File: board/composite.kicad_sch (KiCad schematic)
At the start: 18 parts, among them J6 COMPOSITE, U17 CPST, U18 74HC373, U19 74HC373, U20 74HC165, U21 74HC165, Y1 14.318MHz

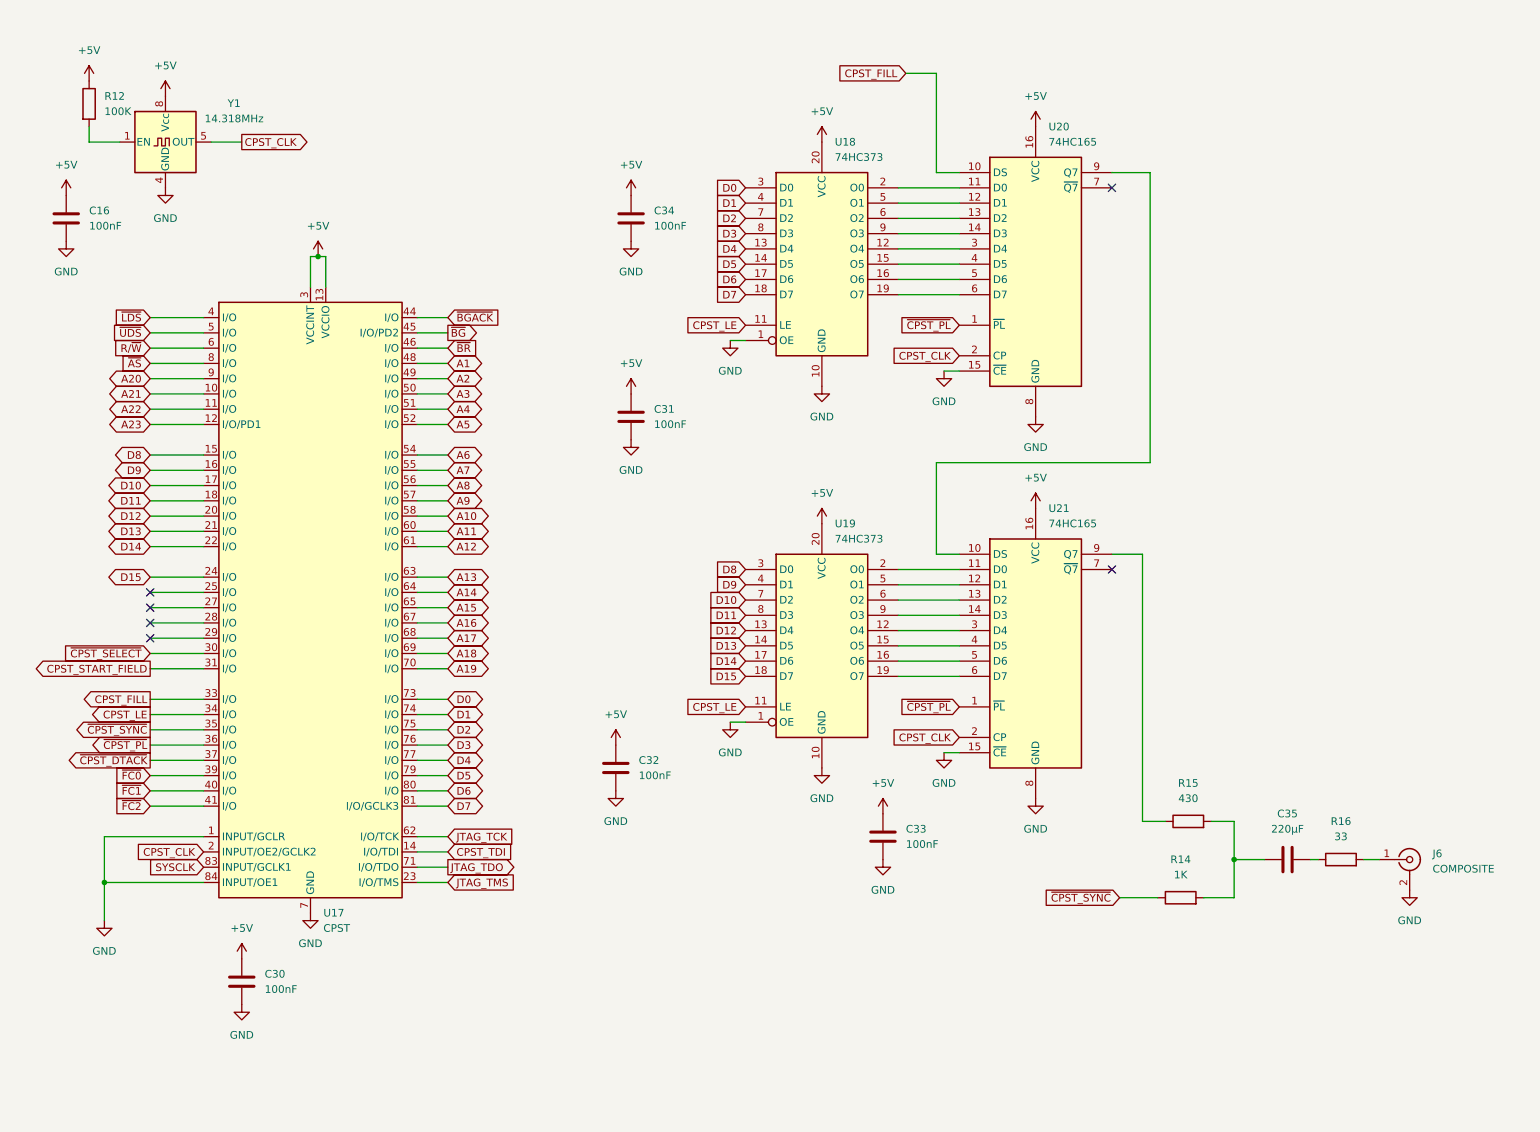
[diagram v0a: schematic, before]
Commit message: checkpoint
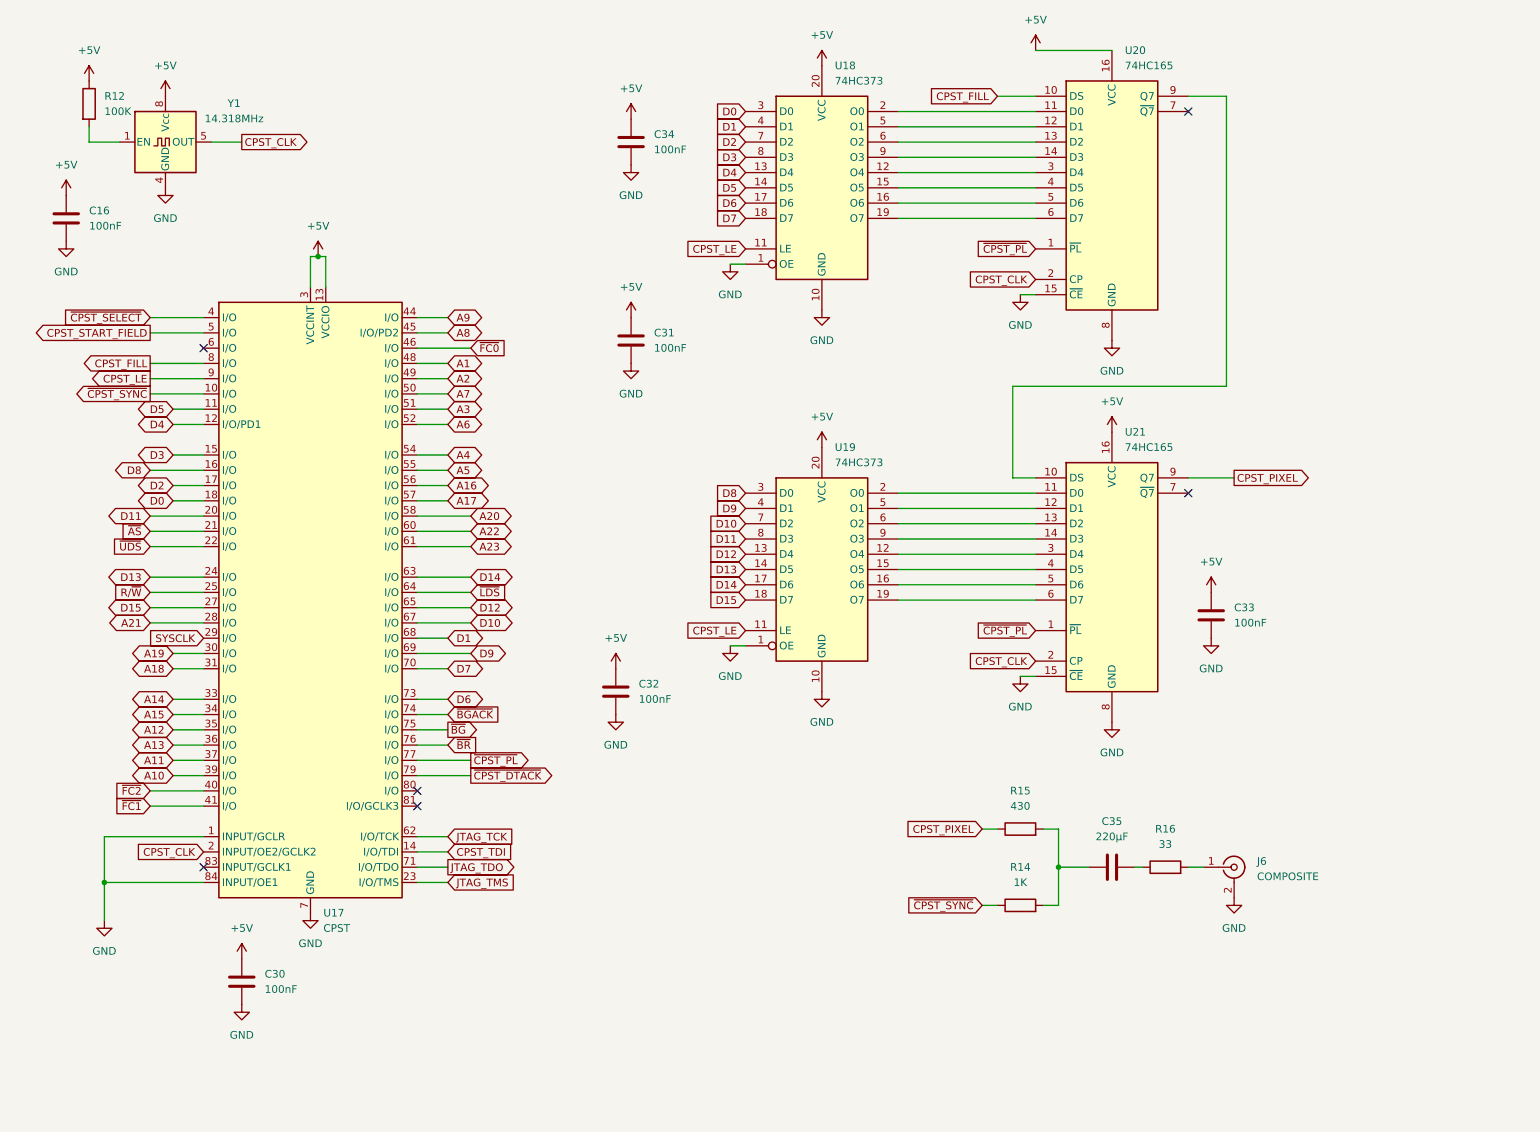
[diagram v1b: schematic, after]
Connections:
- net A10: now also U17.39 (I/O); no longer U17.58 (I/O)
- net A11: now also U17.37 (I/O); no longer U17.60 (I/O)
- net A12: now also U17.35 (I/O); no longer U17.61 (I/O)
- net A13: now also U17.36 (I/O); no longer U17.63 (I/O)
- net A14: now also U17.33 (I/O); no longer U17.64 (I/O)
- net A15: now also U17.34 (I/O); no longer U17.65 (I/O)
- net A16: now also U17.56 (I/O); no longer U17.67 (I/O)
- net A17: now also U17.57 (I/O); no longer U17.68 (I/O)
- net A18: now also U17.31 (I/O); no longer U17.69 (I/O)
- net A19: now also U17.30 (I/O); no longer U17.70 (I/O)
- net A20: now also U17.58 (I/O); no longer U17.9 (I/O)
- net A21: now also U17.28 (I/O); no longer U17.10 (I/O)
- net A22: now also U17.60 (I/O); no longer U17.11 (I/O)
- net A23: now also U17.61 (I/O); no longer U17.12 (I/O/PD1)
- net A3: now also U17.51 (I/O); no longer U17.50 (I/O)
- net A4: now also U17.54 (I/O); no longer U17.51 (I/O)
- net A5: now also U17.55 (I/O); no longer U17.52 (I/O)
- net A6: now also U17.52 (I/O); no longer U17.54 (I/O)
- net A7: now also U17.50 (I/O); no longer U17.55 (I/O)
- net A8: now also U17.45 (I/O/PD2); no longer U17.56 (I/O)
- net A9: now also U17.44 (I/O); no longer U17.57 (I/O)
- net CPST_FILL: now also U17.8 (I/O); no longer U17.33 (I/O)
- net CPST_LE: now also U17.9 (I/O); no longer U17.34 (I/O)
- net CPST_START_FIELD: now also U17.5 (I/O); no longer U17.31 (I/O)
- net D0: now also U17.18 (I/O); no longer U17.73 (I/O)
- net D1: now also U17.68 (I/O); no longer U17.74 (I/O)
- net D10: now also U17.67 (I/O); no longer U17.17 (I/O)
- net D11: now also U17.20 (I/O); no longer U17.18 (I/O)
- net D12: now also U17.65 (I/O); no longer U17.20 (I/O)
- net D13: now also U17.24 (I/O); no longer U17.21 (I/O)
- net D14: now also U17.63 (I/O); no longer U17.22 (I/O)
- net D15: now also U17.27 (I/O); no longer U17.24 (I/O)
- net D2: now also U17.17 (I/O); no longer U17.75 (I/O)
- net D3: now also U17.15 (I/O); no longer U17.76 (I/O)
- net D4: now also U17.12 (I/O/PD1); no longer U17.77 (I/O)
- net D5: now also U17.11 (I/O); no longer U17.79 (I/O)
- net D6: now also U17.73 (I/O); no longer U17.80 (I/O)
- net D7: now also U17.70 (I/O); no longer U17.81 (I/O/GCLK3)
- net D8: now also U17.16 (I/O); no longer U17.15 (I/O)
- net D9: now also U17.69 (I/O); no longer U17.16 (I/O)
- net R/~{W}: now also U17.25 (I/O); no longer U17.6 (I/O)
- net SYSCLK: now also U17.29 (I/O); no longer U17.83 (INPUT/GCLK1)
- net ~{AS}: now also U17.21 (I/O); no longer U17.8 (I/O)
- net ~{BGACK}: now also U17.74 (I/O); no longer U17.44 (I/O)
- net ~{BG}: now also U17.75 (I/O); no longer U17.45 (I/O/PD2)
- net ~{BR}: now also U17.76 (I/O); no longer U17.46 (I/O)
- net ~{CPST_DTACK}: now also U17.79 (I/O); no longer U17.37 (I/O)
- net ~{CPST_PL}: now also U17.77 (I/O); no longer U17.36 (I/O)
- net ~{CPST_SELECT}: now also U17.4 (I/O); no longer U17.30 (I/O)
- net ~{CPST_SYNC}: now also U17.10 (I/O); no longer U17.35 (I/O)
- net ~{FC0}: now also U17.46 (I/O); no longer U17.39 (I/O)
- net ~{FC1}: now also U17.41 (I/O); no longer U17.40 (I/O)
- net ~{FC2}: now also U17.40 (I/O); no longer U17.41 (I/O)
- net ~{LDS}: now also U17.64 (I/O); no longer U17.4 (I/O)
- net ~{UDS}: now also U17.22 (I/O); no longer U17.5 (I/O)
- net CPST_PIXEL: now reaches R15.1, U21.9 (Q7)
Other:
- moved on the sheet: C31, C32, C33, C34, C35, J6, R14, R15, R16, U18, U19, U20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

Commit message: checkpoint before deleting composite video
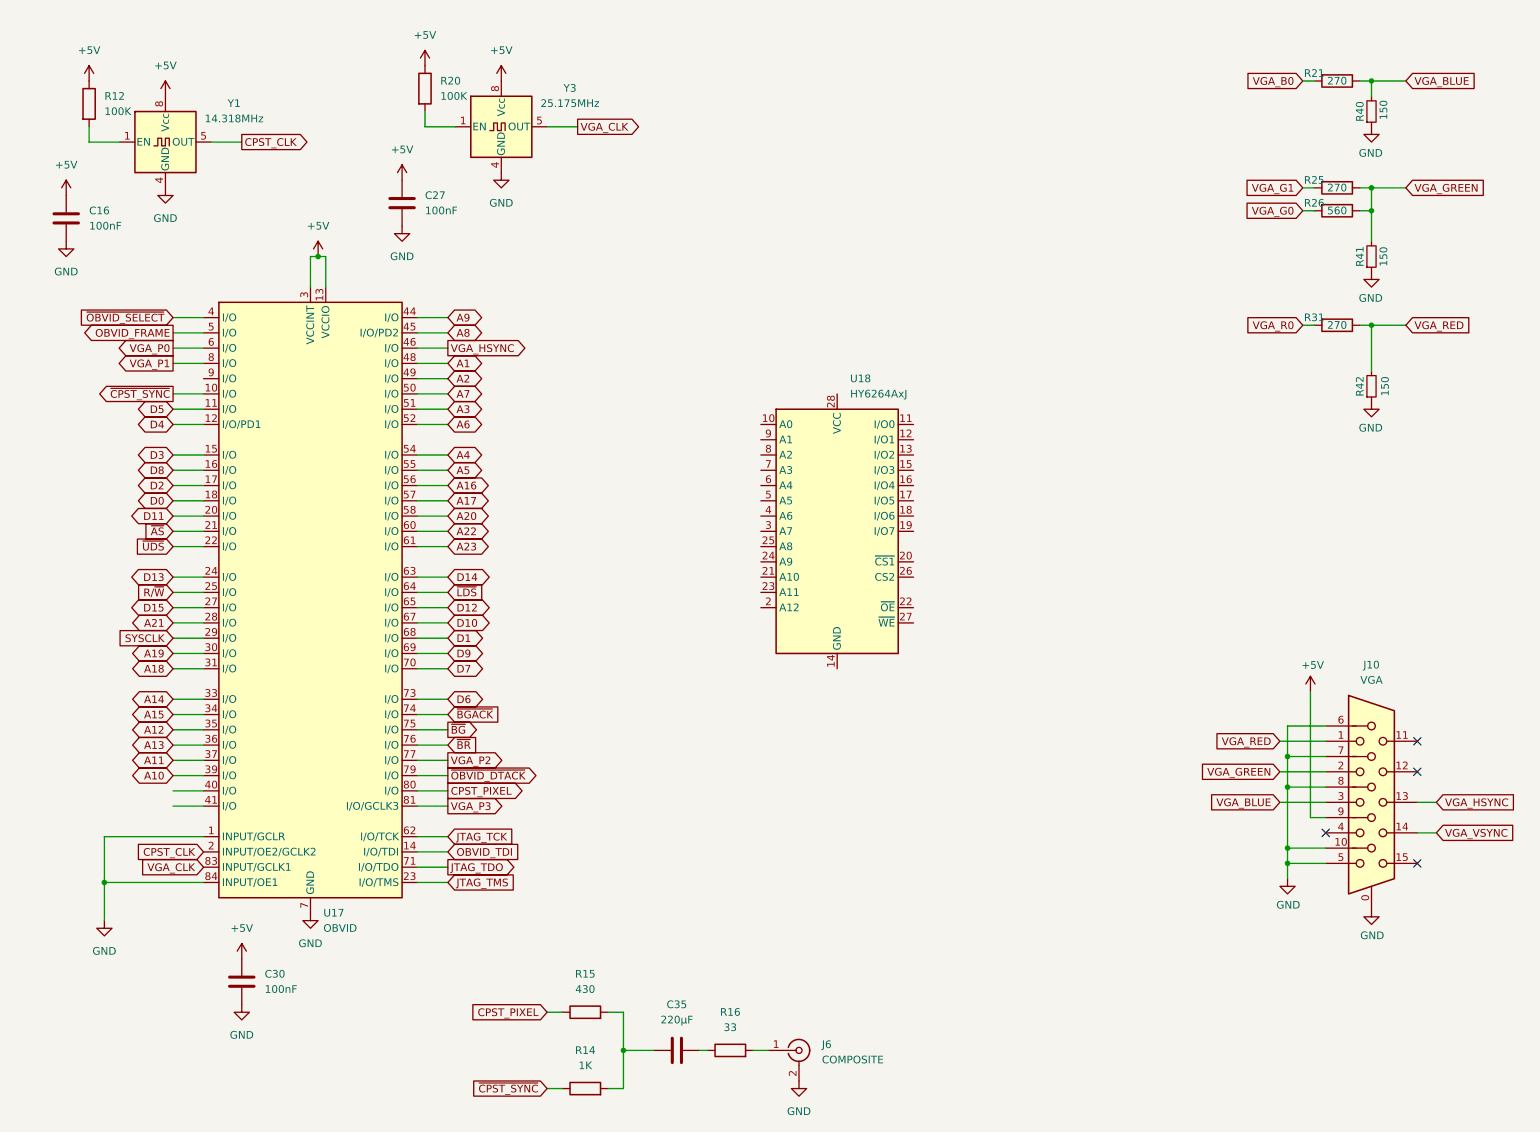
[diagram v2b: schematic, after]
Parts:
- removed C31, C32, C33, C34: 100nF, Capacitor_THT:C_Disc_D5.0mm_W2.5mm_P5.00mm, symbol Device:C
- removed U18, U19: 74HC373, Package_DIP:DIP-20_W7.62mm, symbol 74xx:74HC373
- removed U20, U21: 74HC165, Package_DIP:DIP-16_W7.62mm, symbol 74xx:74HC165
- added C27: 100nF, Capacitor_THT:C_Disc_D5.0mm_W2.5mm_P5.00mm, symbol Device:C
- added J10: VGA, board:HD15-SN-24, symbol Connector:DE15_Socket_HighDensity_MountingHoles
- added R20: 100K, Resistor_THT:R_Axial_DIN0207_L6.3mm_D2.5mm_P10.16mm_Horizontal, symbol Device:R
- added R21, R25, R31: 270, Resistor_THT:R_Axial_DIN0207_L6.3mm_D2.5mm_P10.16mm_Horizontal, symbol Device:R
- added R26: 560, Resistor_THT:R_Axial_DIN0207_L6.3mm_D2.5mm_P10.16mm_Horizontal, symbol Device:R
- added R40, R41, R42: 150, Resistor_THT:R_Axial_DIN0207_L6.3mm_D2.5mm_P10.16mm_Horizontal, symbol Device:R_Small
- added U18: HY6264AxJ, Package_SO:SOP-28_8.4x18.16mm_P1.27mm, symbol Memory_RAM:HY6264AxJ
- added Y3: 25.175MHz, Oscillator:Oscillator_DIP-8, symbol Oscillator:CXO_DIP8
- U17: value CPST -> OBVID
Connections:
- net +5V: now also C27.1, J10.9, R20.1, Y3.8 (Vcc)
- net CPST_PIXEL: now also U17.80 (I/O)
- net GND: now also C27.2, J10.0, J10.10, J10.5, J10.6, J10.7, J10.8, R40.1, R41.1, R42.1, Y3.4 (GND)
- net VGA_P0: now reaches U17.6 (I/O)
- net VGA_P3: now reaches U17.81 (I/O/GCLK3)
- net VGA_CLK: now reaches U17.83 (INPUT/GCLK1)
- net VGA_CLK: now also Y3.5 (OUT)
- net CPST_FILL renamed VGA_P1
- net CPST_LE: no longer names the net of U17.9 (I/O)
- net CPST_START_FIELD renamed OBVID_FRAME
- net CPST_TDI renamed OBVID_TDI
- net ~{CPST_DTACK} renamed ~{OBVID_DTACK}
- net ~{CPST_PL} renamed VGA_P2
- net ~{CPST_SELECT} renamed ~{OBVID_SELECT}
- net ~{FC0} renamed VGA_HSYNC
- net VGA_HSYNC: now also J10.13
- net ~{FC1}: no longer names the net of U17.41 (I/O)
- net ~{FC2}: no longer names the net of U17.40 (I/O)
- new net: R20.2, Y3.1 (EN)
- new net VGA_B0: R21.2
- new net VGA_BLUE: J10.3, R21.1, R40.2
- new net VGA_G0: R26.2
- new net VGA_G1: R25.2
- new net VGA_GREEN: J10.2, R25.1, R26.1, R41.2
- new net VGA_R0: R31.2
- new net VGA_RED: J10.1, R31.1, R42.2
- new net VGA_VSYNC: J10.14
- no-connect marks 6 -> 4
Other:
- moved on the sheet: C35, J6, R14, R15, R16

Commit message: checkpoint before compact flash
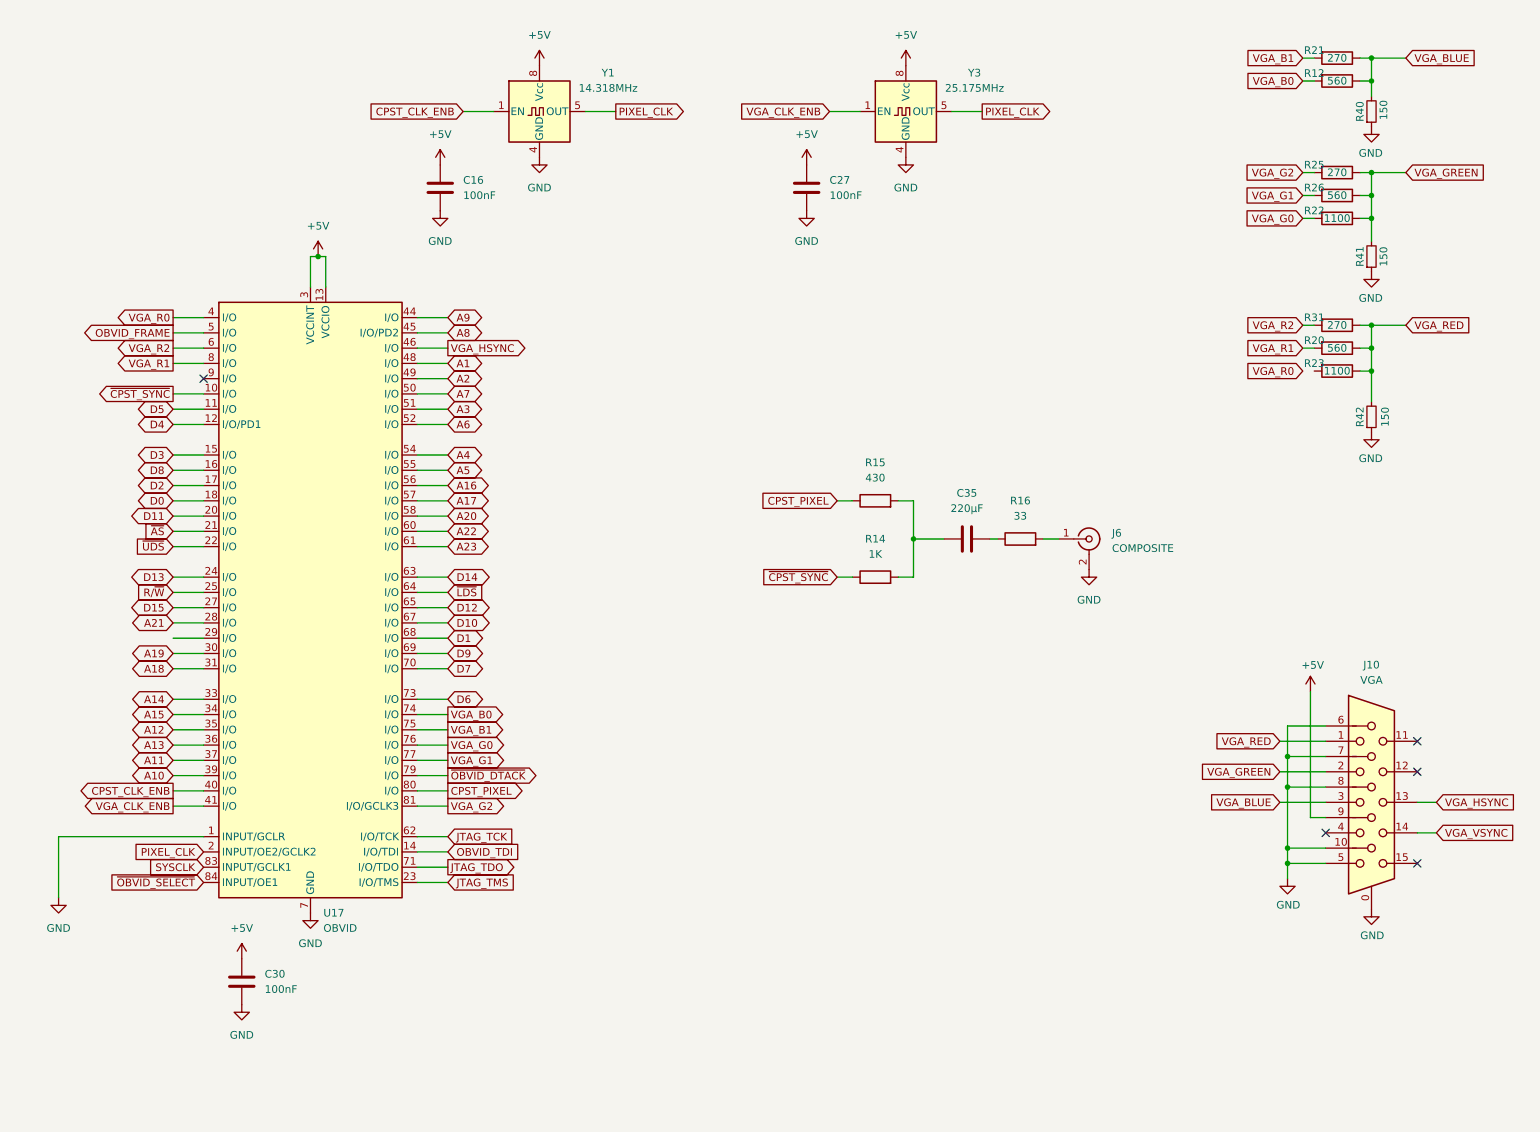
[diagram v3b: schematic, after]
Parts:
- removed U18: HY6264AxJ, Package_SO:SOP-28_8.4x18.16mm_P1.27mm, symbol Memory_RAM:HY6264AxJ
- added R22, R23: 1100, Resistor_SMD:R_0603_1608Metric, symbol Device:R
- R12, R20: value 100K -> 560; Package (none) -> 0603; Type (none) -> SMD
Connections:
- net VGA_P2 is gone; now on net VGA_G1: U17.77 (I/O)
- net ~{BGACK} is gone; now on net VGA_B0: U17.74 (I/O)
- net ~{BR} is gone; now on net VGA_G0: U17.76 (I/O)
- net +5V: no longer R12.1, R20.1
- net GND: no longer U17.84 (INPUT/OE1)
- net SYSCLK: now also U17.83 (INPUT/GCLK1); no longer U17.29 (I/O)
- net VGA_B0: now also R12.2; no longer R21.2
- net VGA_BLUE: now also R12.1
- net VGA_G0: now also R22.2; no longer R26.2
- net VGA_G1: now also R26.2; no longer R25.2
- net VGA_GREEN: now also R22.1
- net VGA_R0: now also U17.4 (I/O); no longer R31.2
- net VGA_RED: now also R20.1, R23.1
- net ~{OBVID_SELECT}: now also U17.84 (INPUT/OE1); no longer U17.4 (I/O)
- net VGA_CLK_ENB: now reaches Y3.1 (EN)
- net VGA_CLK_ENB: now also U17.41 (I/O); no longer R20.2
- net CPST_CLK_ENB: now reaches Y1.1 (EN)
- net CPST_CLK_ENB: now also U17.40 (I/O); no longer R12.2
- net CPST_CLK renamed PIXEL_CLK
- net PIXEL_CLK: now also Y3.5 (OUT)
- removed net VGA_CLK: U17.83 (INPUT/GCLK1), Y3.5 (OUT)
- net VGA_P0 renamed VGA_R2
- net VGA_R2: now also R31.2
- net VGA_P1 renamed VGA_R1
- net VGA_R1: now also R20.2
- net VGA_P3 renamed VGA_G2
- net VGA_G2: now also R25.2
- net ~{BG} renamed VGA_B1
- net VGA_B1: now also R21.2
- no-connect marks 4 -> 5
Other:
- moved on the sheet: C16, C27, C35, J6, R14, R15, R16, R21, R25, R26, R42, Y1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
